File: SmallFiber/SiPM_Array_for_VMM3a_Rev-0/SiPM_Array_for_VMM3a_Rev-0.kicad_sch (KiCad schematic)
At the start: 2 parts

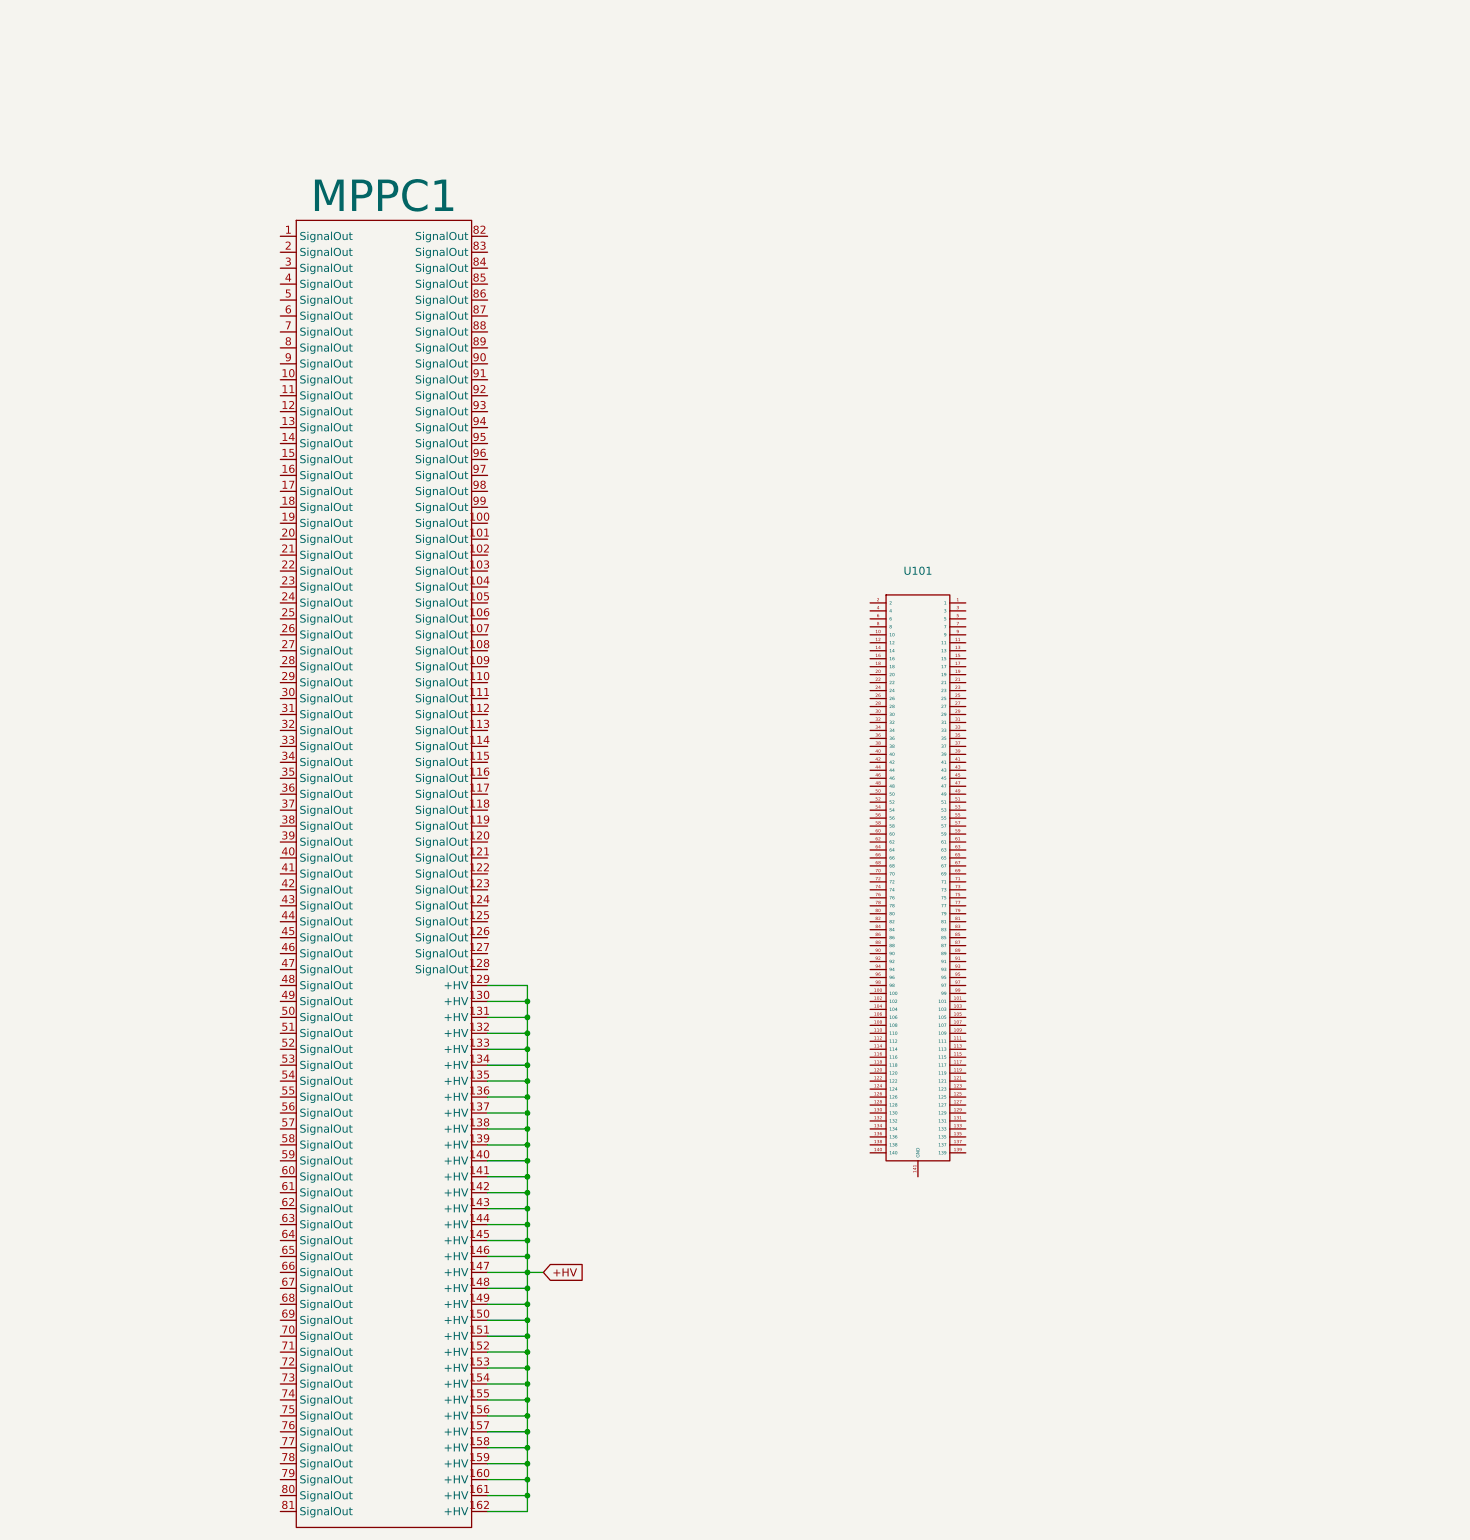
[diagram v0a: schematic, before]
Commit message: .
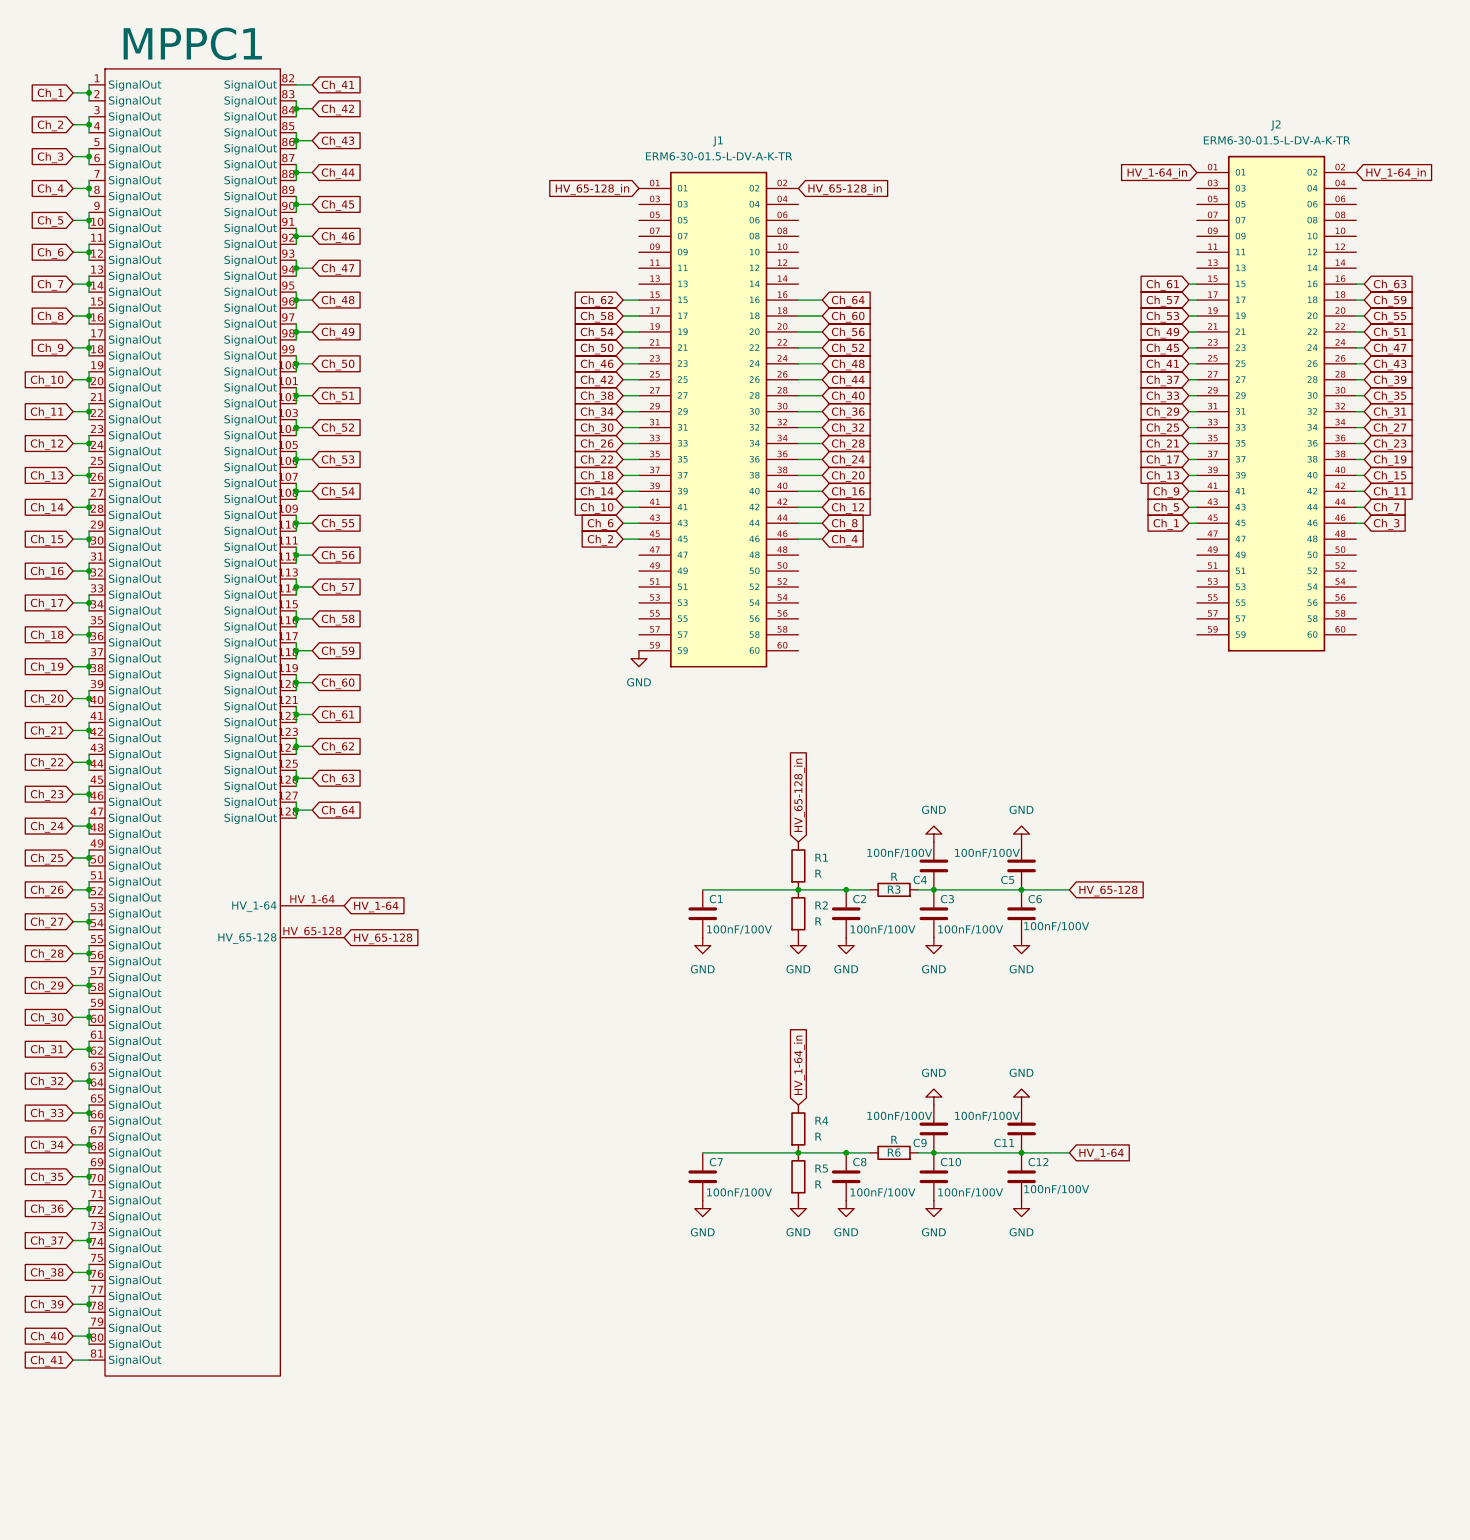
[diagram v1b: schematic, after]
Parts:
- removed U101: ~, 0_lib:Hirose-FX10, symbol 0_FX10-140_Conn:FX10-140
- added C1, C10, C11, C12, C2, C3, C4, C5, C6, C7, C8, C9: 100nF/100V, Capacitor_SMD:C_0201_0603Metric, symbol Device:C
- added J1, J2: ERM6-30-01.5-L-DV-A-K-TR, 0_lib:SAMTEC_ERM6-30-01.5-L-DV-A-K-TR, symbol 0_Samtec_ERM6:ERM6-30-01.5-L-DV-A-K-TR
- added R1, R2, R3, R4, R5, R6: R, Resistor_SMD:R_0201_0603Metric, symbol Device:R
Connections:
- net Ch_1: now reaches MPPC1.1 (SignalOut)
- net Ch_1: now also MPPC1.2 (SignalOut), J2.45
- net Ch_5: now reaches MPPC1.10 (SignalOut)
- net Ch_5: now also MPPC1.9 (SignalOut), J2.43
- net Ch_50: now reaches MPPC1.100 (SignalOut)
- net Ch_50: now also MPPC1.99 (SignalOut), J1.21
- net Ch_51: now reaches MPPC1.101 (SignalOut)
- net Ch_51: now also MPPC1.102 (SignalOut), J2.22
- net Ch_52: now reaches MPPC1.103 (SignalOut)
- net Ch_52: now also MPPC1.104 (SignalOut), J1.22
- net Ch_53: now reaches MPPC1.105 (SignalOut)
- net Ch_53: now also MPPC1.106 (SignalOut), J2.19
- net Ch_54: now reaches MPPC1.107 (SignalOut)
- net Ch_54: now also MPPC1.108 (SignalOut), J1.19
- net Ch_55: now reaches MPPC1.109 (SignalOut)
- net Ch_55: now also MPPC1.110 (SignalOut), J2.20
- net Ch_6: now reaches MPPC1.11 (SignalOut)
- net Ch_6: now also MPPC1.12 (SignalOut), J1.43
- net Ch_56: now reaches MPPC1.111 (SignalOut)
- net Ch_56: now also MPPC1.112 (SignalOut), J1.20
- net Ch_57: now reaches MPPC1.113 (SignalOut)
- net Ch_57: now also MPPC1.114 (SignalOut), J2.17
- net Ch_58: now reaches MPPC1.115 (SignalOut)
- net Ch_58: now also MPPC1.116 (SignalOut), J1.17
- net Ch_59: now reaches MPPC1.117 (SignalOut)
- net Ch_59: now also MPPC1.118 (SignalOut), J2.18
- net Ch_60: now reaches MPPC1.119 (SignalOut)
- net Ch_60: now also MPPC1.120 (SignalOut), J1.18
- net Ch_61: now reaches MPPC1.121 (SignalOut)
- net Ch_61: now also MPPC1.122 (SignalOut), J2.15
- net Ch_62: now reaches MPPC1.123 (SignalOut)
- net Ch_62: now also MPPC1.124 (SignalOut), J1.15
- net Ch_63: now reaches MPPC1.125 (SignalOut)
- net Ch_63: now also MPPC1.126 (SignalOut), J2.16
- net Ch_64: now reaches MPPC1.127 (SignalOut)
- net Ch_64: now also MPPC1.128 (SignalOut), J1.16
- net Ch_7: now reaches MPPC1.13 (SignalOut)
- net Ch_7: now also MPPC1.14 (SignalOut), J2.44
- net Ch_8: now reaches MPPC1.15 (SignalOut)
- net Ch_8: now also MPPC1.16 (SignalOut), J1.44
- net Ch_9: now reaches MPPC1.17 (SignalOut)
- net Ch_9: now also MPPC1.18 (SignalOut), J2.41
- net Ch_10: now reaches MPPC1.19 (SignalOut)
- net Ch_10: now also MPPC1.20 (SignalOut), J1.41
- net Ch_11: now reaches MPPC1.21 (SignalOut)
- net Ch_11: now also MPPC1.22 (SignalOut), J2.42
- net Ch_12: now reaches MPPC1.23 (SignalOut)
- net Ch_12: now also MPPC1.24 (SignalOut), J1.42
- net Ch_13: now reaches MPPC1.25 (SignalOut)
- net Ch_13: now also MPPC1.26 (SignalOut), J2.39
- net Ch_14: now reaches MPPC1.27 (SignalOut)
- net Ch_14: now also MPPC1.28 (SignalOut), J1.39
- net Ch_15: now reaches MPPC1.29 (SignalOut)
- net Ch_15: now also MPPC1.30 (SignalOut), J2.40
- net Ch_2: now reaches MPPC1.3 (SignalOut)
- net Ch_2: now also MPPC1.4 (SignalOut), J1.45
- net Ch_16: now reaches MPPC1.31 (SignalOut)
- net Ch_16: now also MPPC1.32 (SignalOut), J1.40
- net Ch_17: now reaches MPPC1.33 (SignalOut)
- net Ch_17: now also MPPC1.34 (SignalOut), J2.37
- net Ch_18: now reaches MPPC1.35 (SignalOut)
- net Ch_18: now also MPPC1.36 (SignalOut), J1.37
- net Ch_19: now reaches MPPC1.37 (SignalOut)
- net Ch_19: now also MPPC1.38 (SignalOut), J2.38
- net Ch_20: now reaches MPPC1.39 (SignalOut)
- net Ch_20: now also MPPC1.40 (SignalOut), J1.38
- net Ch_21: now reaches MPPC1.41 (SignalOut)
- net Ch_21: now also MPPC1.42 (SignalOut), J2.35
- net Ch_22: now reaches MPPC1.43 (SignalOut)
- net Ch_22: now also MPPC1.44 (SignalOut), J1.35
- net Ch_23: now reaches MPPC1.45 (SignalOut)
- net Ch_23: now also MPPC1.46 (SignalOut), J2.36
- net Ch_24: now reaches MPPC1.47 (SignalOut)
- net Ch_24: now also MPPC1.48 (SignalOut), J1.36
- net Ch_25: now reaches MPPC1.49 (SignalOut)
- net Ch_25: now also MPPC1.50 (SignalOut), J2.33
- net Ch_3: now reaches MPPC1.5 (SignalOut)
- net Ch_3: now also MPPC1.6 (SignalOut), J2.46
- net Ch_26: now reaches MPPC1.51 (SignalOut)
- net Ch_26: now also MPPC1.52 (SignalOut), J1.33
- net Ch_27: now reaches MPPC1.53 (SignalOut)
- net Ch_27: now also MPPC1.54 (SignalOut), J2.34
- net Ch_28: now reaches MPPC1.55 (SignalOut)
- net Ch_28: now also MPPC1.56 (SignalOut), J1.34
- net Ch_29: now reaches MPPC1.57 (SignalOut)
- net Ch_29: now also MPPC1.58 (SignalOut), J2.31
- net Ch_30: now reaches MPPC1.59 (SignalOut)
- net Ch_30: now also MPPC1.60 (SignalOut), J1.31
- net Ch_31: now reaches MPPC1.61 (SignalOut)
- net Ch_31: now also MPPC1.62 (SignalOut), J2.32
- net Ch_32: now reaches MPPC1.63 (SignalOut)
- net Ch_32: now also MPPC1.64 (SignalOut), J1.32
- net Ch_33: now reaches MPPC1.65 (SignalOut)
- net Ch_33: now also MPPC1.66 (SignalOut), J2.29
- net Ch_34: now reaches MPPC1.67 (SignalOut)
- net Ch_34: now also MPPC1.68 (SignalOut), J1.29
- net Ch_35: now reaches MPPC1.69 (SignalOut)
- net Ch_35: now also MPPC1.70 (SignalOut), J2.30
- net Ch_4: now reaches MPPC1.7 (SignalOut)
- net Ch_4: now also MPPC1.8 (SignalOut), J1.46
- net Ch_36: now reaches MPPC1.71 (SignalOut)
- net Ch_36: now also MPPC1.72 (SignalOut), J1.30
- net Ch_37: now reaches MPPC1.73 (SignalOut)
- net Ch_37: now also MPPC1.74 (SignalOut), J2.27
- net Ch_38: now reaches MPPC1.75 (SignalOut)
- net Ch_38: now also MPPC1.76 (SignalOut), J1.27
- net Ch_39: now reaches MPPC1.77 (SignalOut)
- net Ch_39: now also MPPC1.78 (SignalOut), J2.28
- net Ch_40: now reaches MPPC1.79 (SignalOut)
- net Ch_40: now also MPPC1.80 (SignalOut), J1.28
- net Ch_41: now reaches MPPC1.81 (SignalOut)
- net Ch_41: now also MPPC1.82 (SignalOut), J2.25
- net Ch_42: now reaches MPPC1.83 (SignalOut)
- net Ch_42: now also MPPC1.84 (SignalOut), J1.25
- net Ch_43: now reaches MPPC1.85 (SignalOut)
- net Ch_43: now also MPPC1.86 (SignalOut), J2.26
- net Ch_44: now reaches MPPC1.87 (SignalOut)
- net Ch_44: now also MPPC1.88 (SignalOut), J1.26
- net Ch_45: now reaches MPPC1.89 (SignalOut)
- net Ch_45: now also MPPC1.90 (SignalOut), J2.23
- net Ch_46: now reaches MPPC1.91 (SignalOut)
- net Ch_46: now also MPPC1.92 (SignalOut), J1.23
- net Ch_47: now reaches MPPC1.93 (SignalOut)
- net Ch_47: now also MPPC1.94 (SignalOut), J2.24
- net Ch_48: now reaches MPPC1.95 (SignalOut)
- net Ch_48: now also MPPC1.96 (SignalOut), J1.24
- net Ch_49: now reaches MPPC1.97 (SignalOut)
- net Ch_49: now also MPPC1.98 (SignalOut), J2.21
- removed net +HV: MPPC1.129 (+HV), MPPC1.130 (+HV), MPPC1.131 (+HV), MPPC1.132 (+HV), MPPC1.133 (+HV), MPPC1.134 (+HV), MPPC1.135 (+HV), MPPC1.136 (+HV), MPPC1.137 (+HV), MPPC1.138 (+HV), MPPC1.139 (+HV), MPPC1.140 (+HV), MPPC1.141 (+HV), MPPC1.142 (+HV), MPPC1.143 (+HV), MPPC1.144 (+HV), MPPC1.145 (+HV), MPPC1.146 (+HV), MPPC1.147 (+HV), MPPC1.148 (+HV), MPPC1.149 (+HV), MPPC1.150 (+HV), MPPC1.151 (+HV), MPPC1.152 (+HV), MPPC1.153 (+HV), MPPC1.154 (+HV), MPPC1.155 (+HV), MPPC1.156 (+HV), MPPC1.157 (+HV), MPPC1.158 (+HV), MPPC1.159 (+HV), MPPC1.160 (+HV), MPPC1.161 (+HV), MPPC1.162 (+HV)
- new net: C7.1, C8.1, R4.2, R5.1, R6.1
- new net: C1.1, C2.1, R1.2, R2.1, R3.1
- new net GND: C1.2, C10.2, C11.2, C12.2, C2.2, C3.2, C4.2, C5.2, C6.2, C7.2, C8.2, C9.2, J1.59, R2.2, R5.2
- new net HV_1-64: C10.1, C11.1, C12.1, C9.1, MPPC1.HV_1-64, R6.2
- new net HV_1-64_in: J2.01, J2.02, R4.1
- new net HV_65-128: C3.1, C4.1, C5.1, C6.1, MPPC1.HV_65-128, R3.2
- new net HV_65-128_in: J1.01, J1.02, R1.1
